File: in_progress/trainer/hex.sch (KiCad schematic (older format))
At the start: 45 parts, among them IC1 ATMEGA16-P, P12 CONN_02X08, P13 CONN_01X02, Q2 2N3904, Q3 2N3904, Q4 2N3904, Q5 2N3904, SW22 DEC/HEX, SW23 SW_PUSH, SW24 SW_PUSH, U10 JHD-162A, U8 4067, U9 ULN2803A

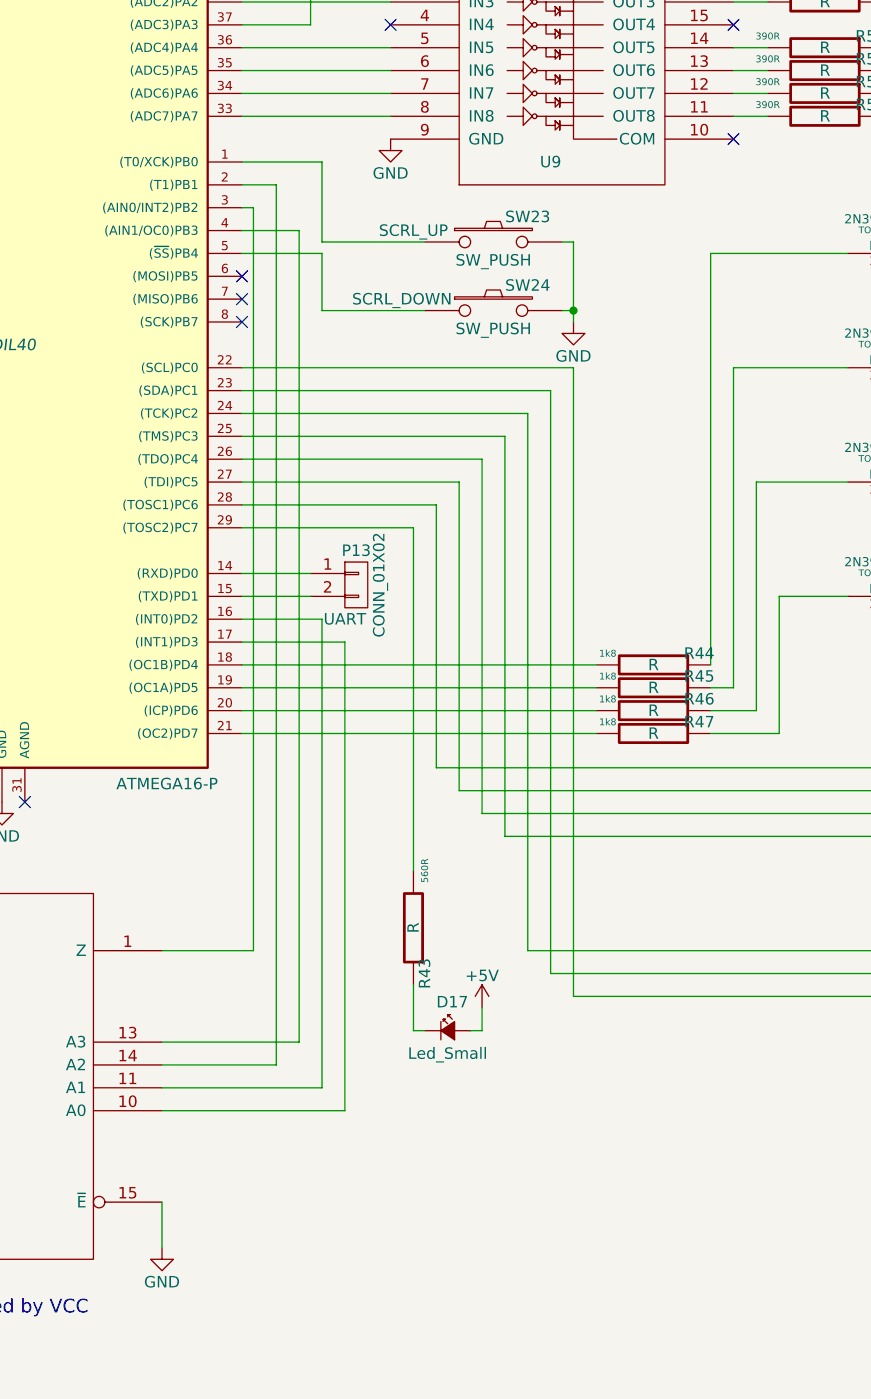
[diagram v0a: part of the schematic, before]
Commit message: .
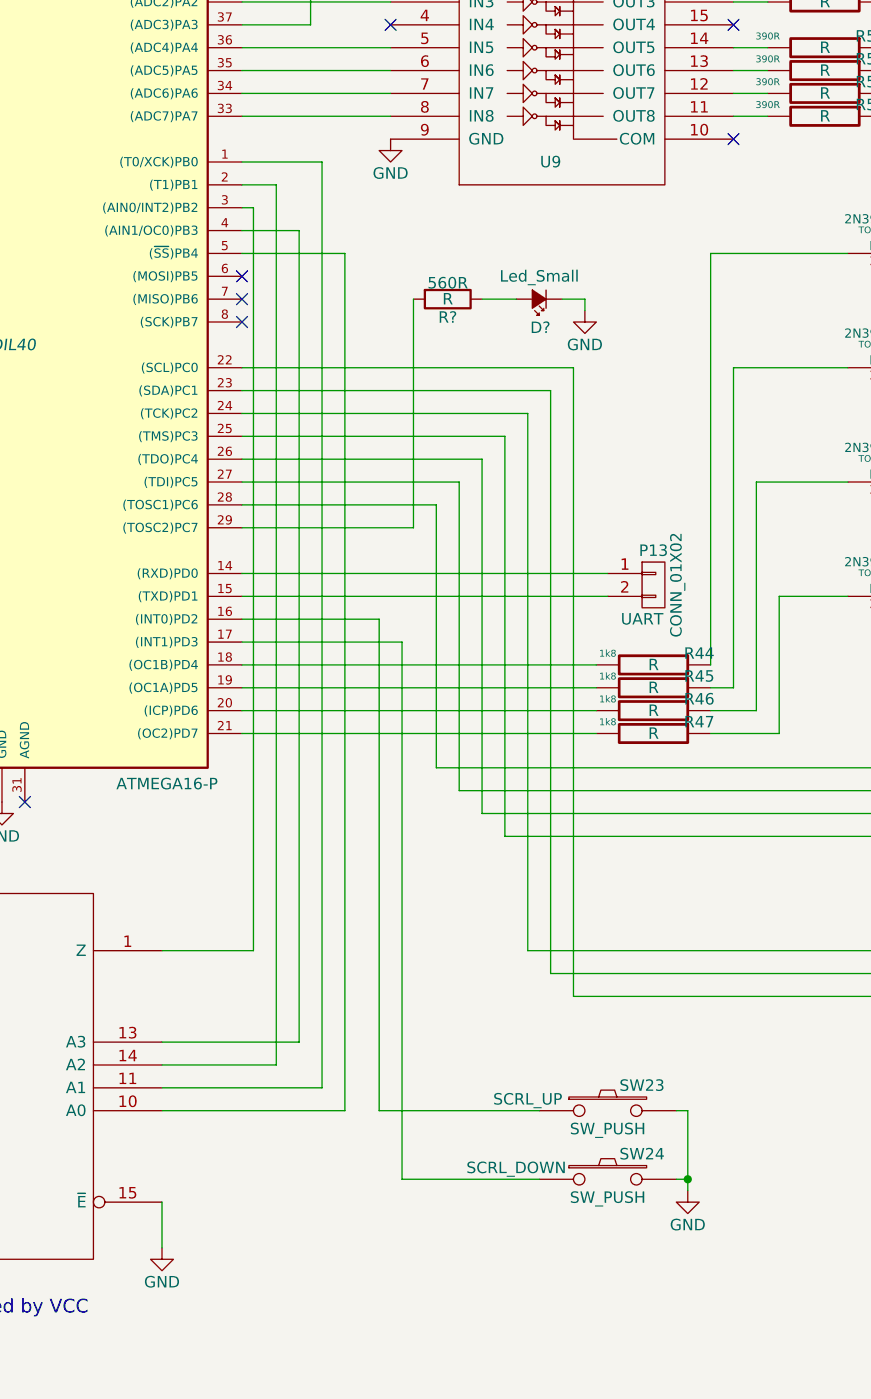
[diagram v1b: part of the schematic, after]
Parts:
- removed D17: Led_Small, symbol Led_Small
- removed R43: R, 560R, symbol R-RESCUE-trainer
- added D?: Led_Small, symbol Led_Small
- added R?: R, 560R, symbol R
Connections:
- net GND: now also D?.1 (K)
- net at U8.10 (A0): now also IC1.5 ((~SS~)PB4); no longer IC1.17 ((INT1)PD3)
- net at U8.11 (A1): now also IC1.1 ((T0/XCK)PB0); no longer IC1.16 ((INT0)PD2)
- net at SW23.1: now also IC1.16 ((INT0)PD2); no longer IC1.1 ((T0/XCK)PB0)
- net at IC1.29 ((TOSC2)PC7): now also R?.2
- net at SW24.1: now also IC1.17 ((INT1)PD3); no longer IC1.5 ((~SS~)PB4)
- new net: D?.2 (A), R?.1
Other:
- moved on the sheet: P13, SW23, SW24
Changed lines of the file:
@@
-$EndComp
-$Comp
-L R-RESCUE-trainer R43
-U 1 1 56687F22
-P 7350 6700
-F 0 "R43" V 7300 6900 50  0000 C CNN
-F 1 "R" V 7350 6700 50  0000 C CNN
-F 2 "560R" V 7300 6450 30  0000 C CNN
-F 3 "" H 7350 6700 30  0000 C CNN
-	1    7350 6700
-	-1   0    0    1
-$EndComp
-$Comp
-L +5V #PWR62
-U 1 1 5668DC41
-P 7650 7050
-F 0 "#PWR62" H 7650 6900 50  0001 C CNN
-F 1 "+5V" H 7650 7190 50  0000 C CNN
-F 2 "" H 7650 7050 50  0000 C CNN
-F 3 "" H 7650 7050 50  0000 C CNN
-	1    7650 7050
-	1    0    0    -1
-$EndComp
-$Comp
-L Led_Small D17
-U 1 1 5668801F
-P 7500 7150
-F 0 "D17" H 7450 7275 50  0000 L CNN
-F 1 "Led_Small" H 7325 7050 50  0000 L CNN
-F 2 "" V 7500 7150 50  0000 C CNN
-F 3 "" V 7500 7150 50  0000 C CNN
-	1    7500 7150
-	1    0    0    -1
 $EndComp
 $Comp
@@
 L CONN_01X02 P13
 U 1 1 5669A8F7
-P 7100 5200
-F 0 "P13" H 7100 5350 50  0000 C CNN
-F 1 "CONN_01X02" V 7200 5200 50  0000 C CNN
-F 2 "UART" H 7050 5050 50  0000 C CNN
-F 3 "" H 7100 5200 50  0000 C CNN
-	1    7100 5200
+P 8400 5200
+F 0 "P13" H 8400 5350 50  0000 C CNN
+F 1 "CONN_01X02" V 8500 5200 50  0000 C CNN
+F 2 "UART" H 8350 5050 50  0000 C CNN
+F 3 "" H 8400 5200 50  0000 C CNN
+	1    8400 5200
 	1    0    0    -1
 $EndComp
@@
 L SW_PUSH SW23
 U 1 1 566A89D8
-P 7700 3700
-F 0 "SW23" H 7850 3810 50  0000 C CNN
-F 1 "SW_PUSH" H 7700 3620 50  0000 C CNN
-F 2 "SCRL_UP" H 7350 3750 50  0000 C CNN
-F 3 "" H 7700 3700 50  0000 C CNN
-	1    7700 3700
+P 8200 7500
+F 0 "SW23" H 8350 7610 50  0000 C CNN
+F 1 "SW_PUSH" H 8200 7420 50  0000 C CNN
+F 2 "SCRL_UP" H 7850 7550 50  0000 C CNN
+F 3 "" H 8200 7500 50  0000 C CNN
+	1    8200 7500
 	1    0    0    -1
 $EndComp
@@
 L SW_PUSH SW24
 U 1 1 566A8AAD
-P 7700 4000
-F 0 "SW24" H 7850 4110 50  0000 C CNN
-F 1 "SW_PUSH" H 7700 3920 50  0000 C CNN
-F 2 "SCRL_DOWN" H 7300 4050 50  0000 C CNN
-F 3 "" H 7700 4000 50  0000 C CNN
-	1    7700 4000
+P 8200 7800
+F 0 "SW24" H 8350 7910 50  0000 C CNN
+F 1 "SW_PUSH" H 8200 7720 50  0000 C CNN
+F 2 "SCRL_DOWN" H 7800 7850 50  0000 C CNN
+F 3 "" H 8200 7800 50  0000 C CNN
+	1    8200 7800
 	1    0    0    -1
 $EndComp
@@
 L GND #PWR64
 U 1 1 566A8FFF
-P 8050 4050
-F 0 "#PWR64" H 8050 3800 50  0001 C CNN
-F 1 "GND" H 8050 3900 50  0000 C CNN
-F 2 "" H 8050 4050 50  0000 C CNN
-F 3 "" H 8050 4050 50  0000 C CNN
-	1    8050 4050
+P 8550 7850
+F 0 "#PWR64" H 8550 7600 50  0001 C CNN
+F 1 "GND" H 8550 7700 50  0000 C CNN
+F 2 "" H 8550 7850 50  0000 C CNN
+F 3 "" H 8550 7850 50  0000 C CNN
+	1    8550 7850
 	1    0    0    -1
 $EndComp
@@
 	12200 4950 11350 4950
 Wire Wire Line
-	7650 7050 7650 7150
-Wire Wire Line
-	7650 7150 7600 7150
-Wire Wire Line
-	7350 4950 7350 6450
-Wire Wire Line
-	7350 6950 7350 7150
-Wire Wire Line
-	7350 7150 7400 7150
-Wire Wire Line
 	11600 7200 12100 7200
 Wire Wire Line
@@
 	6600 3550 6650 3550
 Wire Wire Line
-	6950 5350 6600 5350
-Wire Wire Line
-	7050 5450 6600 5450
-Wire Wire Line
 	6750 7300 6250 7300
 Wire Wire Line
 	6850 7200 6250 7200
 Wire Wire Line
-	6250 7400 6950 7400
-Wire Wire Line
-	6250 7500 7050 7500
+	6950 7400 6250 7400
+Wire Wire Line
+	7050 7500 6250 7500
 Wire Wire Line
 	6600 4250 8050 4250
@@
 	6650 6800 6250 6800
 Wire Wire Line
-	7050 7500 7050 5450
-Wire Wire Line
-	6950 7400 6950 5350
+	7050 3750 7050 7500
+Wire Wire Line
+	6950 3350 6950 7400
 Wire Wire Line
 	6750 3450 6750 7300
@@
 	6600 3650 6850 3650
 Wire Wire Line
-	6600 5150 6900 5150
-Wire Wire Line
-	6600 5250 6900 5250
+	6600 5150 8200 5150
+Wire Wire Line
+	6600 5250 8200 5250
 Wire Wire Line
 	6600 5550 8150 5550
@@
 	6650 3550 6650 6800
 Wire Wire Line
-	6600 3350 6950 3350
-Wire Wire Line
-	6950 3350 6950 3700
-Wire Wire Line
-	6950 3700 7400 3700
-Wire Wire Line
-	6600 3750 6950 3750
-Wire Wire Line
-	6950 3750 6950 4000
-Wire Wire Line
-	6950 4000 7400 4000
-Wire Wire Line
-	8000 4000 8050 4000
-Wire Wire Line
-	8050 3700 8050 4050
-Wire Wire Line
-	8000 3700 8050 3700
-Connection ~ 8050 4000
+	8500 7800 8550 7800
+Wire Wire Line
+	8550 7500 8550 7850
+Wire Wire Line
+	8500 7500 8550 7500
+Connection ~ 8550 7800
+Wire Wire Line
+	6950 3350 6600 3350
+Wire Wire Line
+	7050 3750 6600 3750
+$Comp
+L R R?
+U 1 1 568B24E5
+P 7500 3950
+F 0 "R?" V 7580 3950 50  0000 C CNN
+F 1 "R" V 7500 3950 50  0000 C CNN
+F 2 "560R" V 7430 3950 50  0000 C CNN
+F 3 "" H 7500 3950 50  0000 C CNN
+	1    7500 3950
+	0    1    1    0
+$EndComp
+$Comp
+L Led_Small D?
+U 1 1 568B300A
+P 7900 3950
+F 0 "D?" H 7850 4075 50  0000 L CNN
+F 1 "Led_Small" H 7725 3850 50  0000 L CNN
+F 2 "" V 7900 3950 50  0000 C CNN
+F 3 "" V 7900 3950 50  0000 C CNN
+	1    7900 3950
+	-1   0    0    1
+$EndComp
+$Comp
+L GND #PWR?
+U 1 1 568B30CE
+P 8100 4000
+F 0 "#PWR?" H 8100 3750 50  0001 C CNN
+F 1 "GND" H 8100 3850 50  0000 C CNN
+F 2 "" H 8100 4000 50  0000 C CNN
+F 3 "" H 8100 4000 50  0000 C CNN
+	1    8100 4000
+	1    0    0    -1
+$EndComp
+Wire Wire Line
+	8100 4000 8100 3950
+Wire Wire Line
+	8100 3950 8000 3950
+Wire Wire Line
+	7350 4950 7350 3950
+Wire Wire Line
+	7650 3950 7800 3950
+Wire Wire Line
+	6600 5350 7200 5350
+Wire Wire Line
+	7200 5350 7200 7500
+Wire Wire Line
+	7200 7500 7900 7500
+Wire Wire Line
+	6600 5450 7300 5450
+Wire Wire Line
+	7300 5450 7300 7800
+Wire Wire Line
+	7300 7800 7900 7800
 $EndSCHEMATC
